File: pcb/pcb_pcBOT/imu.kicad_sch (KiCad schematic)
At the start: 3 parts, among them U601 LSM6DSM

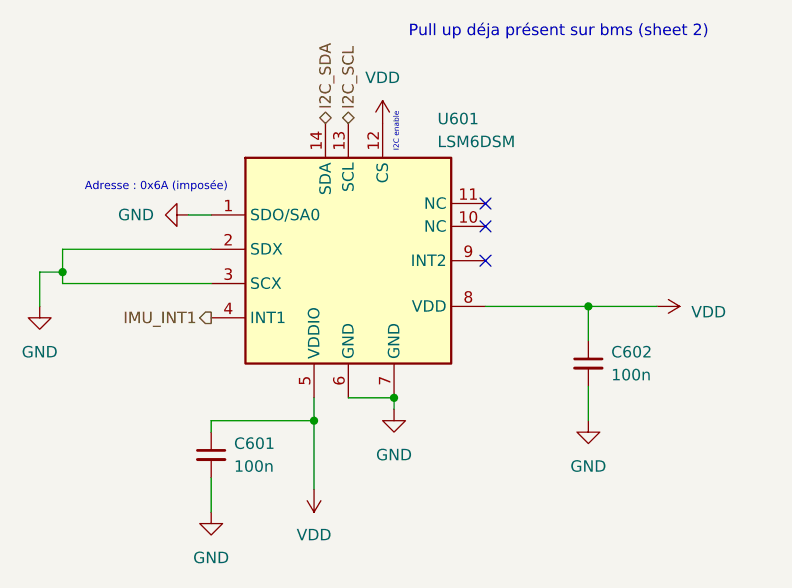
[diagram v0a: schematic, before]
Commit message: Revert "Ajout empreintes (incomplet) + test erc correct"
This reverts commit 267ed5519d67c336b99c9c80b0ac2067182b82a3.
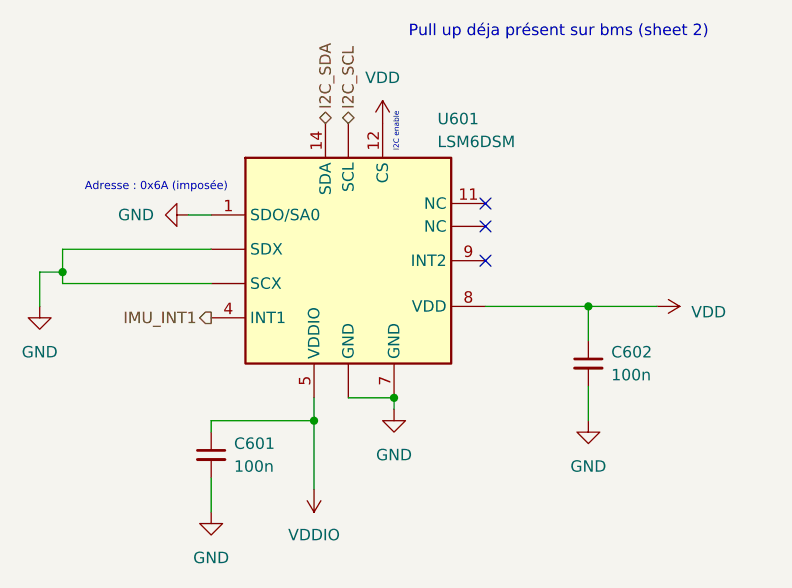
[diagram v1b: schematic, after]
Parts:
- C601, C602: footprint Capacitor_SMD:C_0805_2012Metric_Pad1.18x1.45mm_HandSolder -> (none)
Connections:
- net GND: now also U601. (NC); no longer U601.2 (SDX), U601.3 (SCX), U601.6 (GND)
- net I2C_SCL: now also U601. (NC); no longer U601.13 (SCL)
- net VDD: no longer C601.1, U601.5 (VDDIO)
- new net VDDIO: C601.1, U601.5 (VDDIO)
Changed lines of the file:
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@@
 	(symbol
 		(lib_id "power:VDD")
+		(at 189.23 83.82 270)
+		(unit 1)
+		(exclude_from_sim no)
+		(in_bom yes)
+		(on_board yes)
+		(dnp no)
+		(fields_autoplaced yes)
+		(property "Reference" "#PWR0605"
+			(at 185.42 83.82 0)
+			(effects
+				(font
+					(size 1.27 1.27)
+				)
+				(hide yes)
+			)
+		)
+		(property "Value" "VDD"
+			(at 193.04 84.455 90)
+			(effects
+				(font
+					(size 1.27 1.27)
+				)
+				(justify left)
+			)
+		)
+		(property "Footprint" ""
+			(at 189.23 83.82 0)
+			(effects
+				(font
+					(size 1.27 1.27)
+				)
+				(hide yes)
+			)
+		)
+		(property "Datasheet" ""
+			(at 189.23 83.82 0)
+			(effects
+				(font
+					(size 1.27 1.27)
+				)
+				(hide yes)
+			)
+		)
+		(property "Description" "Power symbol creates a global label with name \"VDD\""
+			(at 189.23 83.82 0)
+			(effects
+				(font
+					(size 1.27 1.27)
+				)
+				(hide yes)
+			)
+		)
+		(pin "1"
+		)
+		(instances
+			(project "pcb_pcBOT"
+				(path "/704e4da3-8ee7-458f-8a0f-3fc97e8dc2a6/ccd57063-24ab-4973-bd12-151ee600ad9c"
+					(reference "#PWR0605")
+					(unit 1)
+				)
+			)
+		)
+	)
+	(symbol
+		(lib_id "power:GND")
+		(at 137.16 73.66 270)
+		(unit 1)
+		(exclude_from_sim no)
+		(in_bom yes)
+		(on_board yes)
+		(dnp no)
+		(fields_autoplaced yes)
+		(property "Reference" "#PWR0607"
+			(at 130.81 73.66 0)
+			(effects
+				(font
+					(size 1.27 1.27)
+				)
+				(hide yes)
+			)
+		)
+		(property "Value" "GND"
+			(at 133.35 73.6599 90)
+			(effects
+				(font
+					(size 1.27 1.27)
+				)
+				(justify right)
+			)
+		)
+		(property "Footprint" ""
+			(at 137.16 73.66 0)
+			(effects
+				(font
+					(size 1.27 1.27)
+				)
+				(hide yes)
+			)
+		)
+		(property "Datasheet" ""
+			(at 137.16 73.66 0)
+			(effects
+				(font
+					(size 1.27 1.27)
+				)
+				(hide yes)
+			)
+		)
+		(property "Description" "Power symbol creates a global label with name \"GND\" , ground"
+			(at 137.16 73.66 0)
+			(effects
+				(font
+					(size 1.27 1.27)
+				)
+				(hide yes)
+			)
+		)
+		(pin "1"
+		)
+		(instances
+			(project ""
+				(path "/704e4da3-8ee7-458f-8a0f-3fc97e8dc2a6/ccd57063-24ab-4973-bd12-151ee600ad9c"
+					(reference "#PWR0607")
+					(unit 1)
+				)
+			)
+		)
+	)
+	(symbol
+		(lib_id "power:VCC")
 		(at 151.13 104.14 180)
 		(unit 1)
@@
 			)
 		)
-		(property "Value" "VDD"
+		(property "Value" "VDDIO"
 			(at 151.13 109.22 0)
 			(effects
@@
 			)
 		)
-		(property "Description" "Power symbol creates a global label with name \"VDD\""
+		(property "Description" "Power symbol creates a global label with name \"VCC\""
 			(at 151.13 104.14 0)
 			(effects
@@
 				(path "/704e4da3-8ee7-458f-8a0f-3fc97e8dc2a6/ccd57063-24ab-4973-bd12-151ee600ad9c"
 					(reference "#PWR0603")
-					(unit 1)
-				)
-			)
-		)
-	)
-	(symbol
-		(lib_id "power:VDD")
-		(at 189.23 83.82 270)
-		(unit 1)
-		(exclude_from_sim no)
-		(in_bom yes)
-		(on_board yes)
-		(dnp no)
-		(fields_autoplaced yes)
-		(property "Reference" "#PWR0605"
-			(at 185.42 83.82 0)
-			(effects
-				(font
-					(size 1.27 1.27)
-				)
-				(hide yes)
-			)
-		)
-		(property "Value" "VDD"
-			(at 193.04 84.455 90)
-			(effects
-				(font
-					(size 1.27 1.27)
-				)
-				(justify left)
-			)
-		)
-		(property "Footprint" ""
-			(at 189.23 83.82 0)
-			(effects
-				(font
-					(size 1.27 1.27)
-				)
-				(hide yes)
-			)
-		)
-		(property "Datasheet" ""
-			(at 189.23 83.82 0)
-			(effects
-				(font
-					(size 1.27 1.27)
-				)
-				(hide yes)
-			)
-		)
-		(property "Description" "Power symbol creates a global label with name \"VDD\""
-			(at 189.23 83.82 0)
-			(effects
-				(font
-					(size 1.27 1.27)
-				)
-				(hide yes)
-			)
-		)
-		(pin "1"
-		)
-		(instances
-			(project "pcb_pcBOT"
-				(path "/704e4da3-8ee7-458f-8a0f-3fc97e8dc2a6/ccd57063-24ab-4973-bd12-151ee600ad9c"
-					(reference "#PWR0605")
-					(unit 1)
-				)
-			)
-		)
-	)
-	(symbol
-		(lib_id "power:GND")
-		(at 137.16 73.66 270)
-		(unit 1)
-		(exclude_from_sim no)
-		(in_bom yes)
-		(on_board yes)
-		(dnp no)
-		(fields_autoplaced yes)
-		(property "Reference" "#PWR0607"
-			(at 130.81 73.66 0)
-			(effects
-				(font
-					(size 1.27 1.27)
-				)
-				(hide yes)
-			)
-		)
-		(property "Value" "GND"
-			(at 133.35 73.6599 90)
-			(effects
-				(font
-					(size 1.27 1.27)
-				)
-				(justify right)
-			)
-		)
-		(property "Footprint" ""
-			(at 137.16 73.66 0)
-			(effects
-				(font
-					(size 1.27 1.27)
-				)
-				(hide yes)
-			)
-		)
-		(property "Datasheet" ""
-			(at 137.16 73.66 0)
-			(effects
-				(font
-					(size 1.27 1.27)
-				)
-				(hide yes)
-			)
-		)
-		(property "Description" "Power symbol creates a global label with name \"GND\" , ground"
-			(at 137.16 73.66 0)
-			(effects
-				(font
-					(size 1.27 1.27)
-				)
-				(hide yes)
-			)
-		)
-		(pin "1"
-		)
-		(instances
-			(project ""
-				(path "/704e4da3-8ee7-458f-8a0f-3fc97e8dc2a6/ccd57063-24ab-4973-bd12-151ee600ad9c"
-					(reference "#PWR0607")
 					(unit 1)
 				)
@@
 		(pin "9"
 		)
-		(pin "3"
-		)
-		(pin "10"
-		)
-		(pin "2"
-		)
-		(pin "6"
-		)
-		(pin "13"
+		(pin ""
+		)
+		(pin ""
+		)
+		(pin ""
+		)
+		(pin ""
+		)
+		(pin ""
 		)
 		(instances
@@
 			)
 		)
-		(property "Footprint" "Capacitor_SMD:C_0805_2012Metric_Pad1.18x1.45mm_HandSolder"
+		(property "Footprint" ""
 			(at 181.61 90.17 0)
 			(effects
@@
 			)
 		)
-		(property "Footprint" "Capacitor_SMD:C_0805_2012Metric_Pad1.18x1.45mm_HandSolder"
+		(property "Footprint" ""
 			(at 139.7 100.33 0)
 			(effects
